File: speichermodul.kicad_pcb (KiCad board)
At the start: 2 copper layers, 100 x 160 mm, 66 parts, among them IC1 6116, P1 CONN_3X2, P2 CONN_01X01, P3 CONN_01X01, P4 CONN_01X01, P5 CONN_01X01, P6 CONN_01X01, P7 CONN_01X01, P8 CONN_02X10, P9 CONN_02X10, SW1 SW_PUSH, SW2 SW_PUSH, U1 7400, U2 74LS08, U3 74LS08, U4 74LS14, U5 74LS540, U6 74LS540

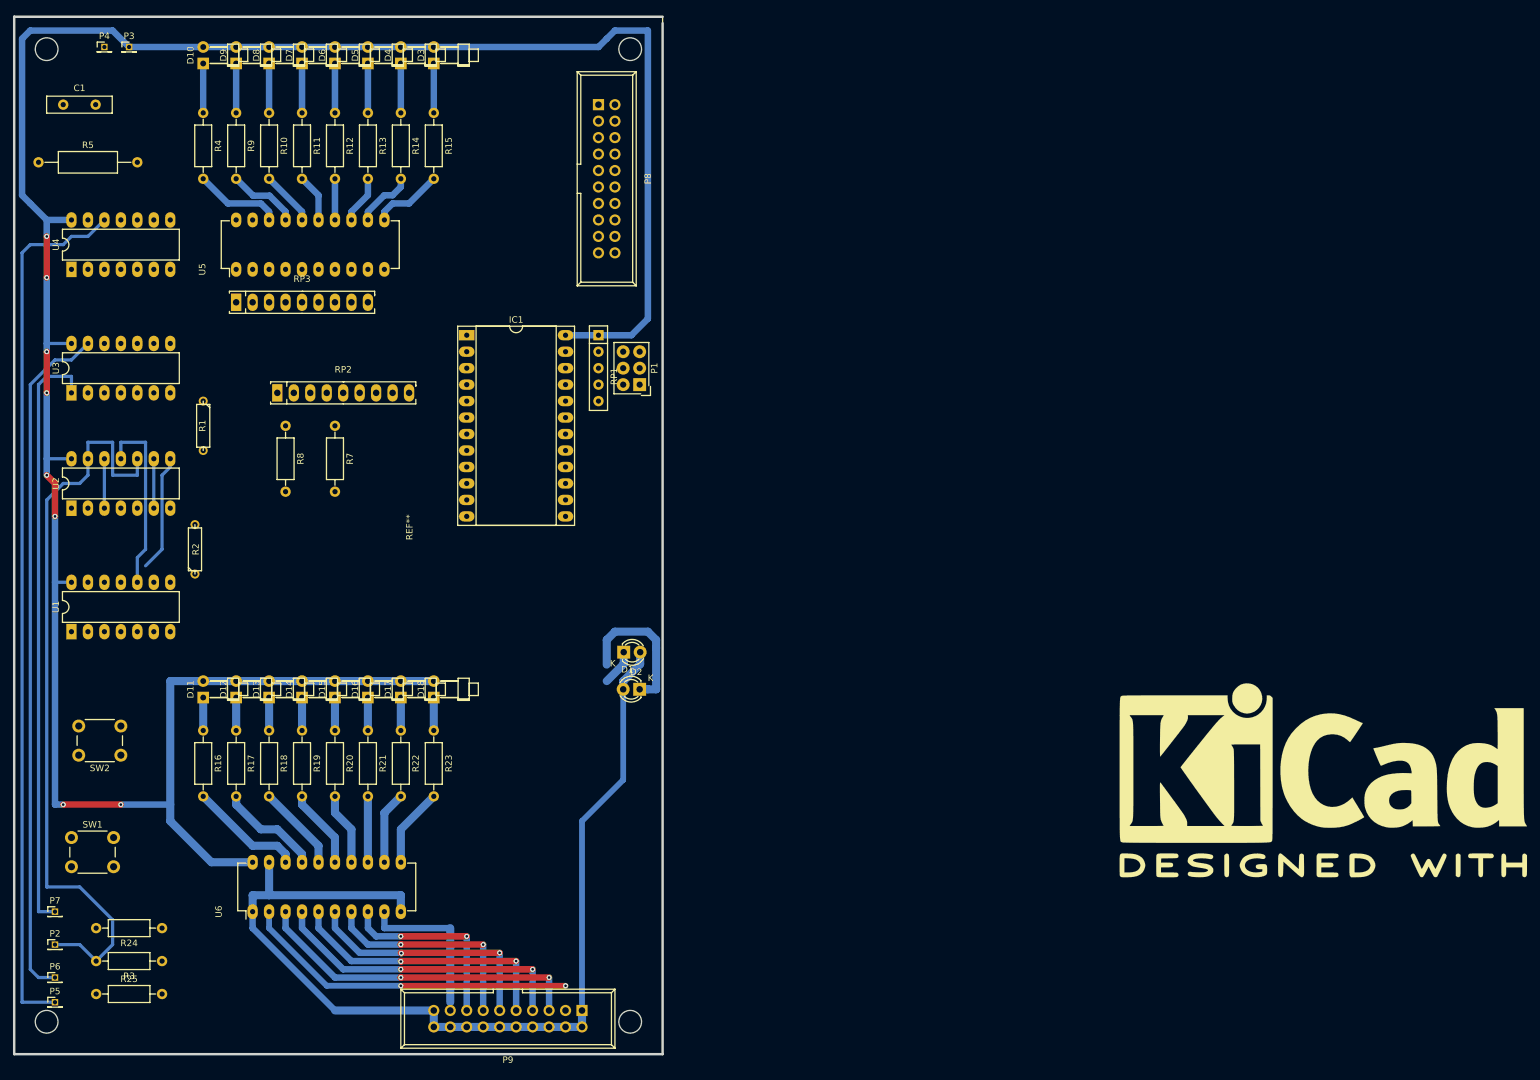
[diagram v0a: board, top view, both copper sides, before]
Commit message: KAel verlegt
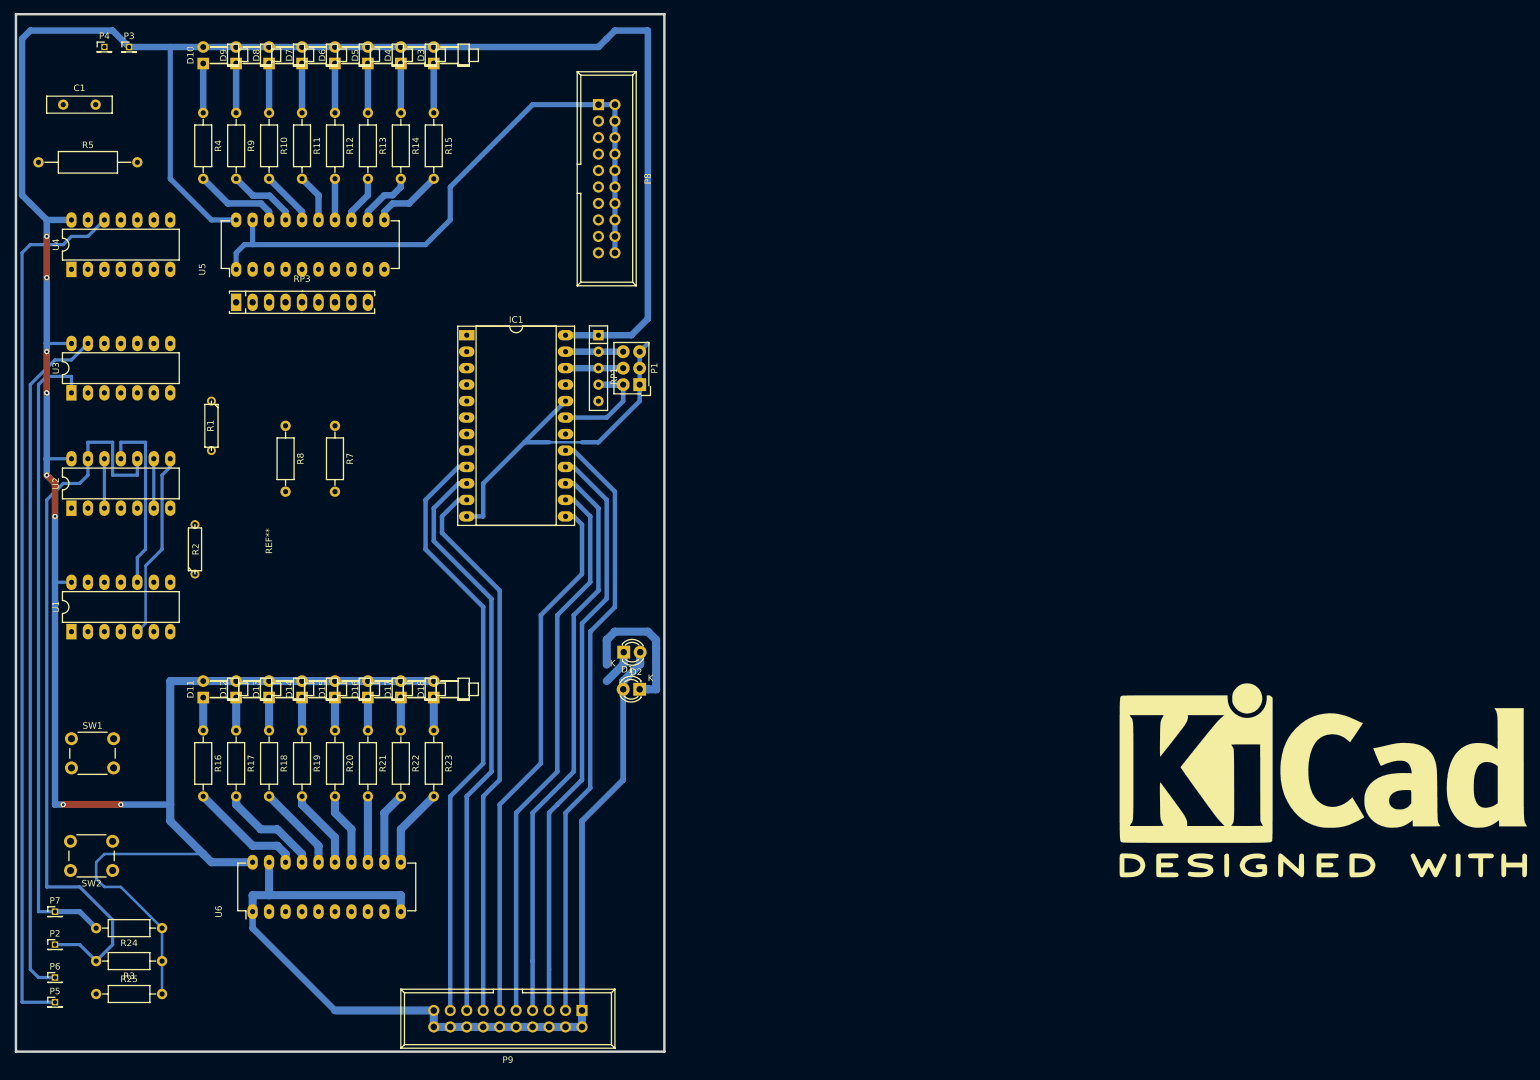
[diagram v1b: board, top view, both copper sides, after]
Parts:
- removed the REF** at (28.0, 22.0)
- removed RP2: R_PACK8BUSSED, Housings_SIP:SIP9_Housing_BigPads
- added REF**: EuroBoard160mmX100mm, EuroBoard_Outline:EuroBoard160mmX100mm, F.Cu at (128.3, 181.6)
- moved SW2 17.8 mm to (43.2, 153.7)
- moved SW1 15.2 mm to (36.8, 133.3)
- moved R1 1.27 mm to (58.4, 85.1)
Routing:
- net GND: track 155.7 -> 311.2 mm
- net /D7: track 0.00 -> 93.4 mm
- net /D0: track 0.00 -> 93.0 mm
- net /D6: track 0.00 -> 90.9 mm
- net /D1: track 0.00 -> 89.4 mm
- net /D5: track 0.00 -> 88.3 mm
- net /D4: track 0.00 -> 85.8 mm
- net /D2: track 0.00 -> 85.8 mm
- net /D3: track 0.00 -> 83.3 mm
- net VCC: track 386.9 -> 463.0 mm
- net /A0: track 51.9 -> 0.00 mm, vias 2 -> 0
- net /A1: track 51.6 -> 0.00 mm, vias 2 -> 0
- net /A2: track 47.1 -> 0.00 mm, vias 2 -> 0
- net /A3: track 42.8 -> 0.00 mm, vias 2 -> 0
- net /A4: track 38.5 -> 0.00 mm, vias 2 -> 0
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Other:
- outline, holes or cut-outs redrawn
- net class Default: trace_width 0.9 -> 0.8
